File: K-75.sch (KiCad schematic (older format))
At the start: 193 parts, among them J1 Conn_01x04, SW1 SW_Push, U1 ATmega32U4-AU, Y1 Crystal_GND24_Small

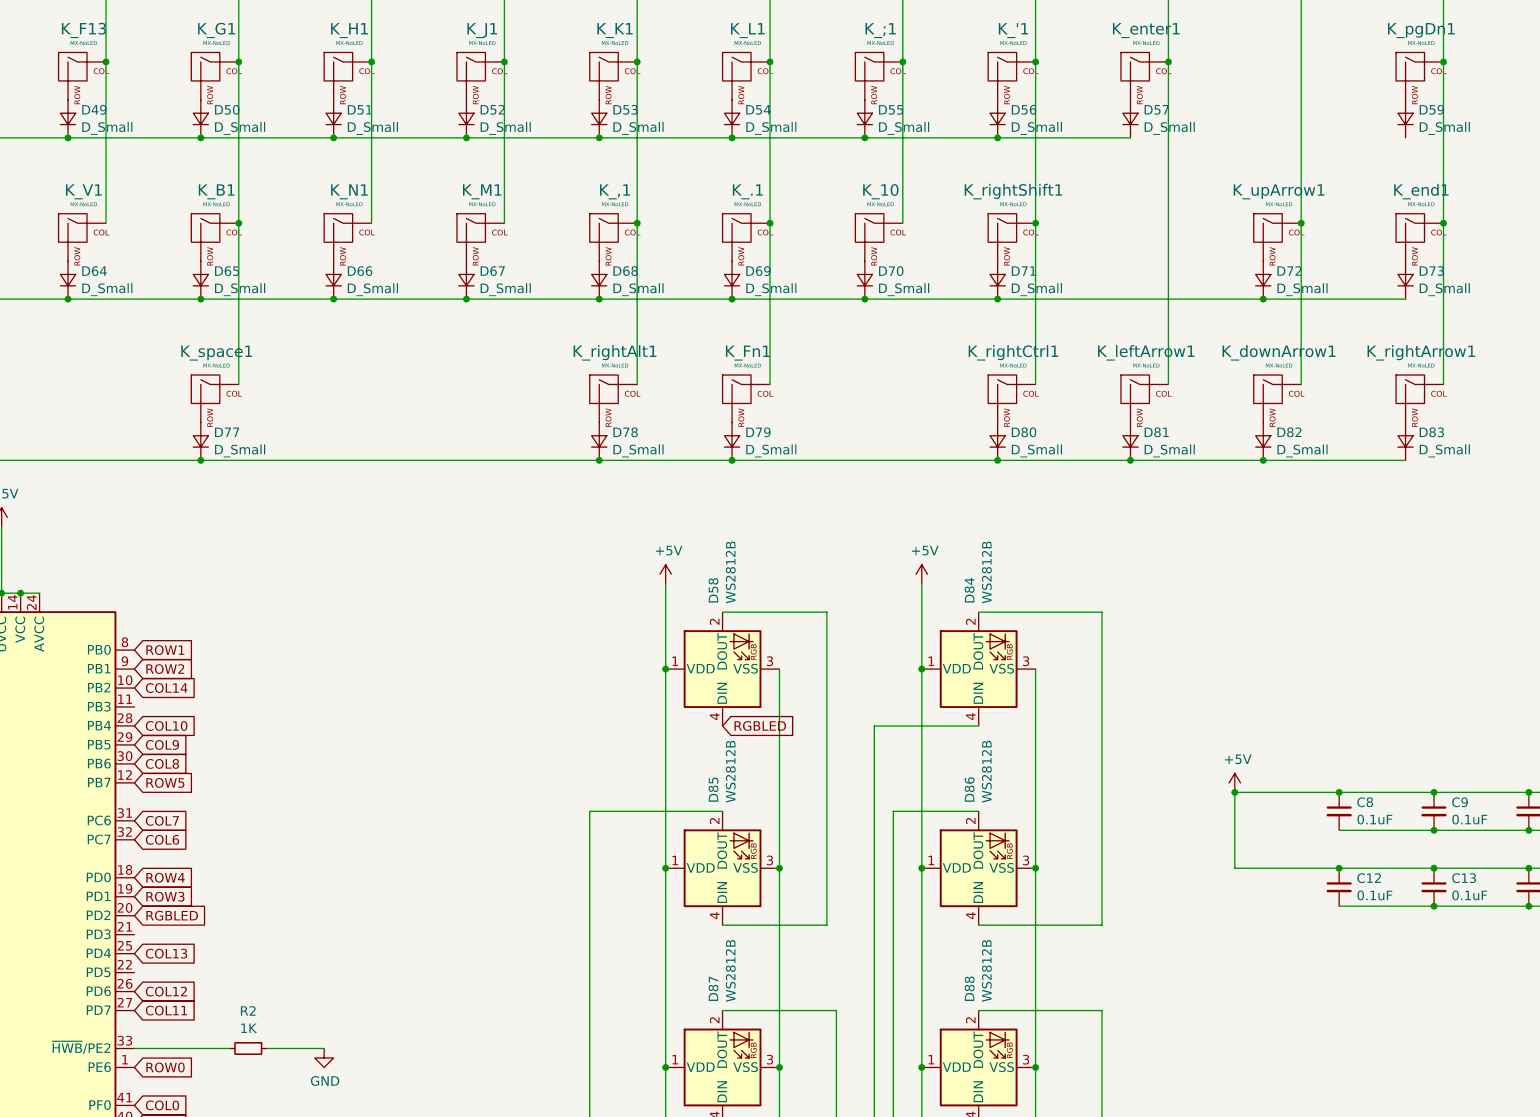
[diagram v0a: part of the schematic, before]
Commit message: Finished routing
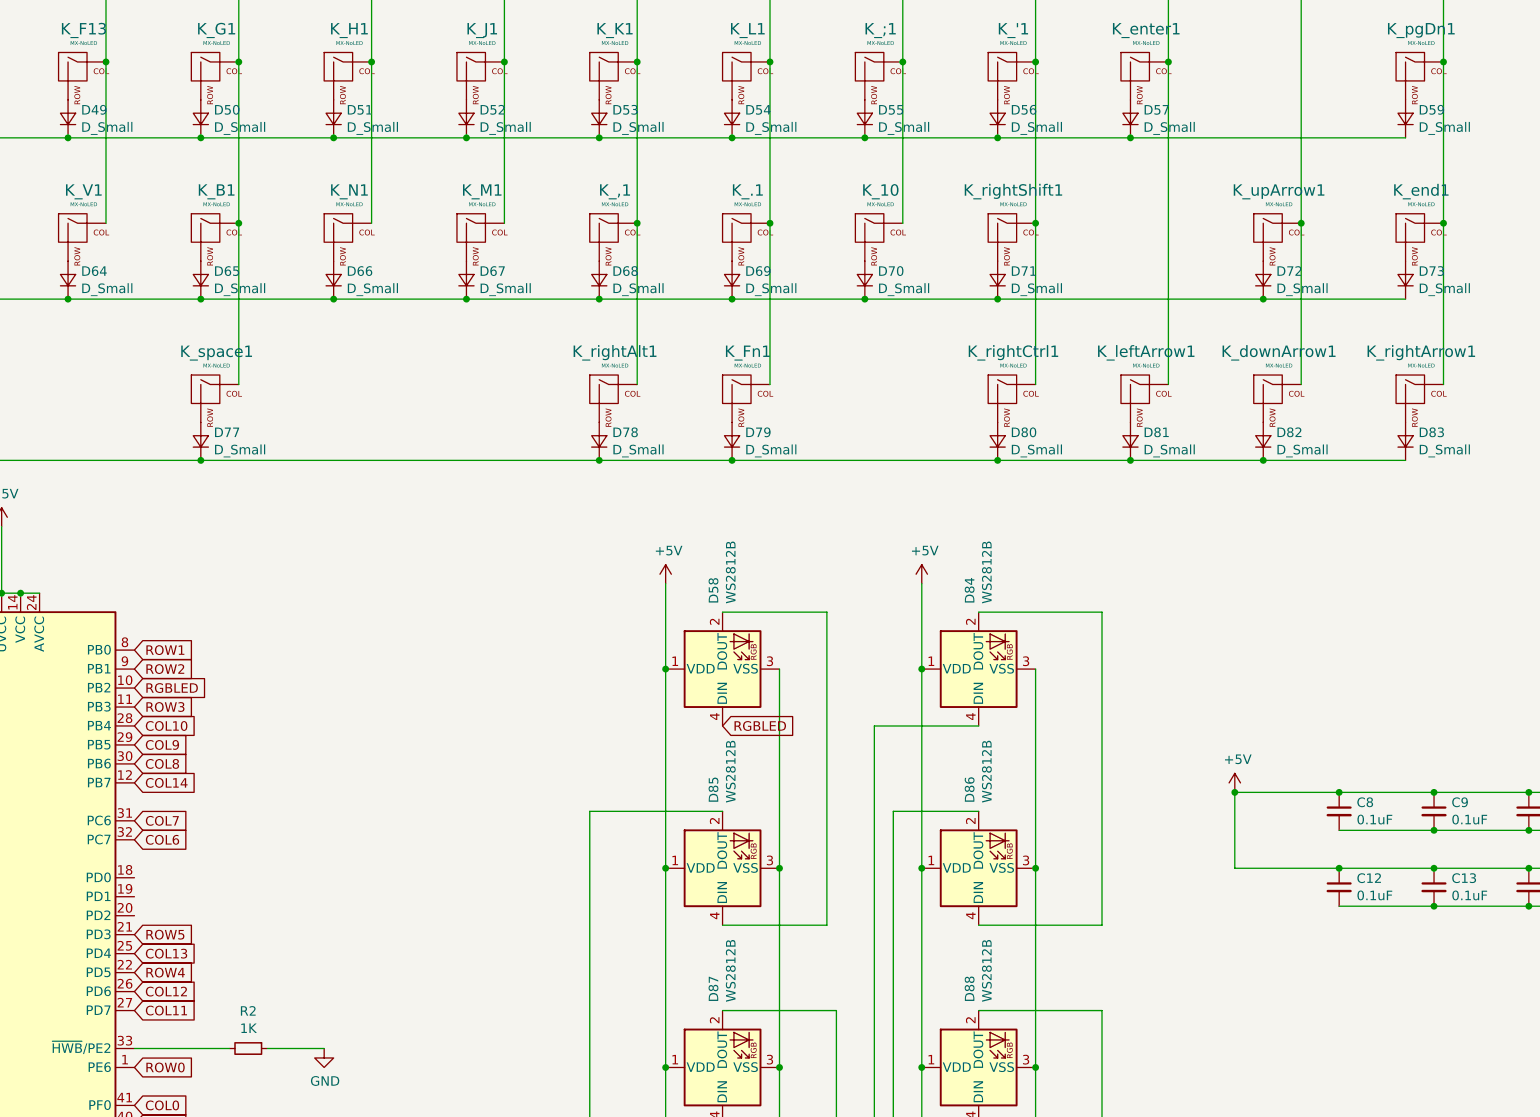
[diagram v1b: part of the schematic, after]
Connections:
- net COL14: now also U1.12 (PB7); no longer U1.10 (PB2)
- net RGBLED: now also U1.10 (PB2); no longer U1.20 (PD2)
- net ROW3: now also D59.1 (K), U1.11 (PB3); no longer U1.19 (PD1)
- net ROW4: now also U1.22 (PD5); no longer U1.18 (PD0)
- net ROW5: now also U1.21 (PD3); no longer U1.12 (PB7)
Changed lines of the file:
@@
 Text GLabel 4750 9850 2    50   Input ~ 0
 COL2
-Text GLabel 4750 9950 2    50   Input ~ 0
-COL3
 Text GLabel 4750 10050 2    50   Input ~ 0
 COL4
@@
 Text GLabel 4750 9050 2    50   Input ~ 0
 COL12
-Text GLabel 4750 8850 2    50   Input ~ 0
-COL13
-Text GLabel 4750 7450 2    50   Input ~ 0
-COL14
 Text GLabel 4750 9450 2    50   Input ~ 0
 ROW0
@@
 Text GLabel 4750 7350 2    50   Input ~ 0
 ROW2
-Text GLabel 4750 8550 2    50   Input ~ 0
+Text GLabel 4750 7550 2    50   Input ~ 0
 ROW3
-Text GLabel 4750 8450 2    50   Input ~ 0
+Text GLabel 4750 8950 2    50   Input ~ 0
 ROW4
-Text GLabel 4750 7950 2    50   Input ~ 0
+Text GLabel 4750 8750 2    50   Input ~ 0
 ROW5
-Text GLabel 4750 8650 2    50   Input ~ 0
-RGBLED
 $Comp
 L LED:WS2812B D58
@@
 $EndComp
 Connection ~ 10550 8000
+Text GLabel 4750 8850 2    50   Input ~ 0
+COL13
+Text GLabel 4750 7450 2    50   Input ~ 0
+RGBLED
+Wire Wire Line
+	10000 4550 11450 4550
+Connection ~ 10000 4550
+Text GLabel 4750 9950 2    50   Input ~ 0
+COL3
+Text GLabel 4750 7950 2    50   Input ~ 0
+COL14
 $EndSCHEMATC
